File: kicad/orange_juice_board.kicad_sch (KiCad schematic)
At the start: 62 parts, among them J10 PWM_OUT1, J11 CONN_UART, J12 PWM_OUT2, J13 FAN_12/24v, J15 PWM_OUT3, J2 DC_INPUT, J3 CONN_ADXL345, J4 OrangePi Zero GPIO PINs, J5 Conn_MAX31865, J7 OrangePi Zero Function Interf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, J8 FAN_5v, J9 PWR_5v, Q1 AO4407A, Q2 AO3400A, Q3 AO3400A, Q4 AO3400A, U1 MP2315GJ-Z

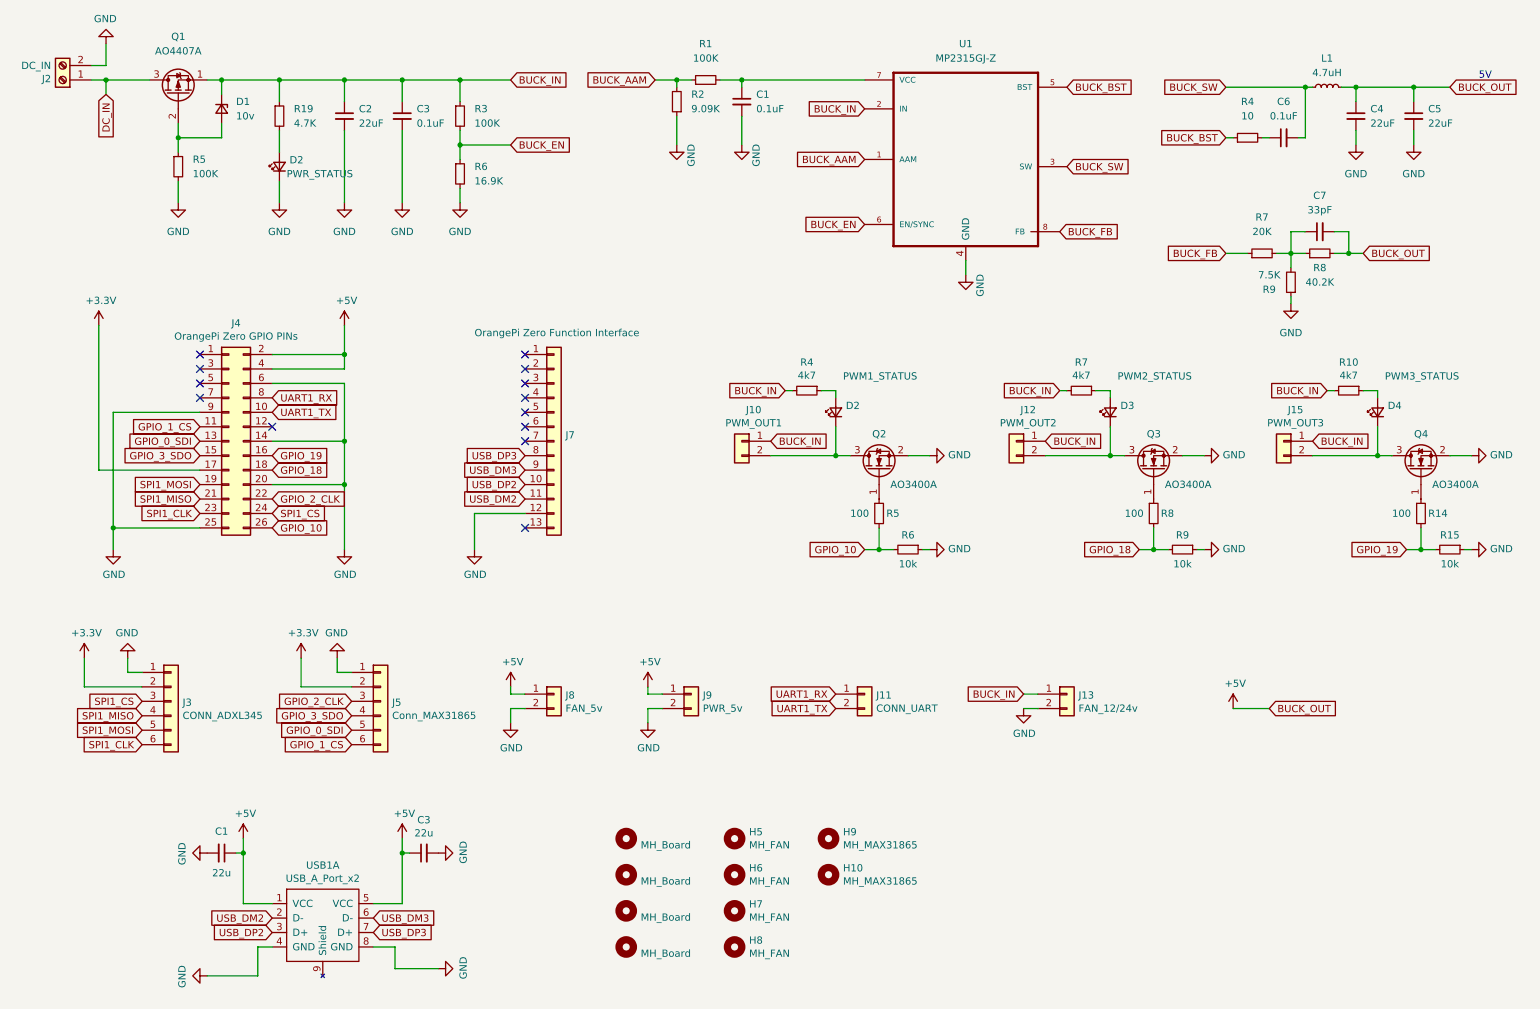
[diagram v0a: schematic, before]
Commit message: update v0.6
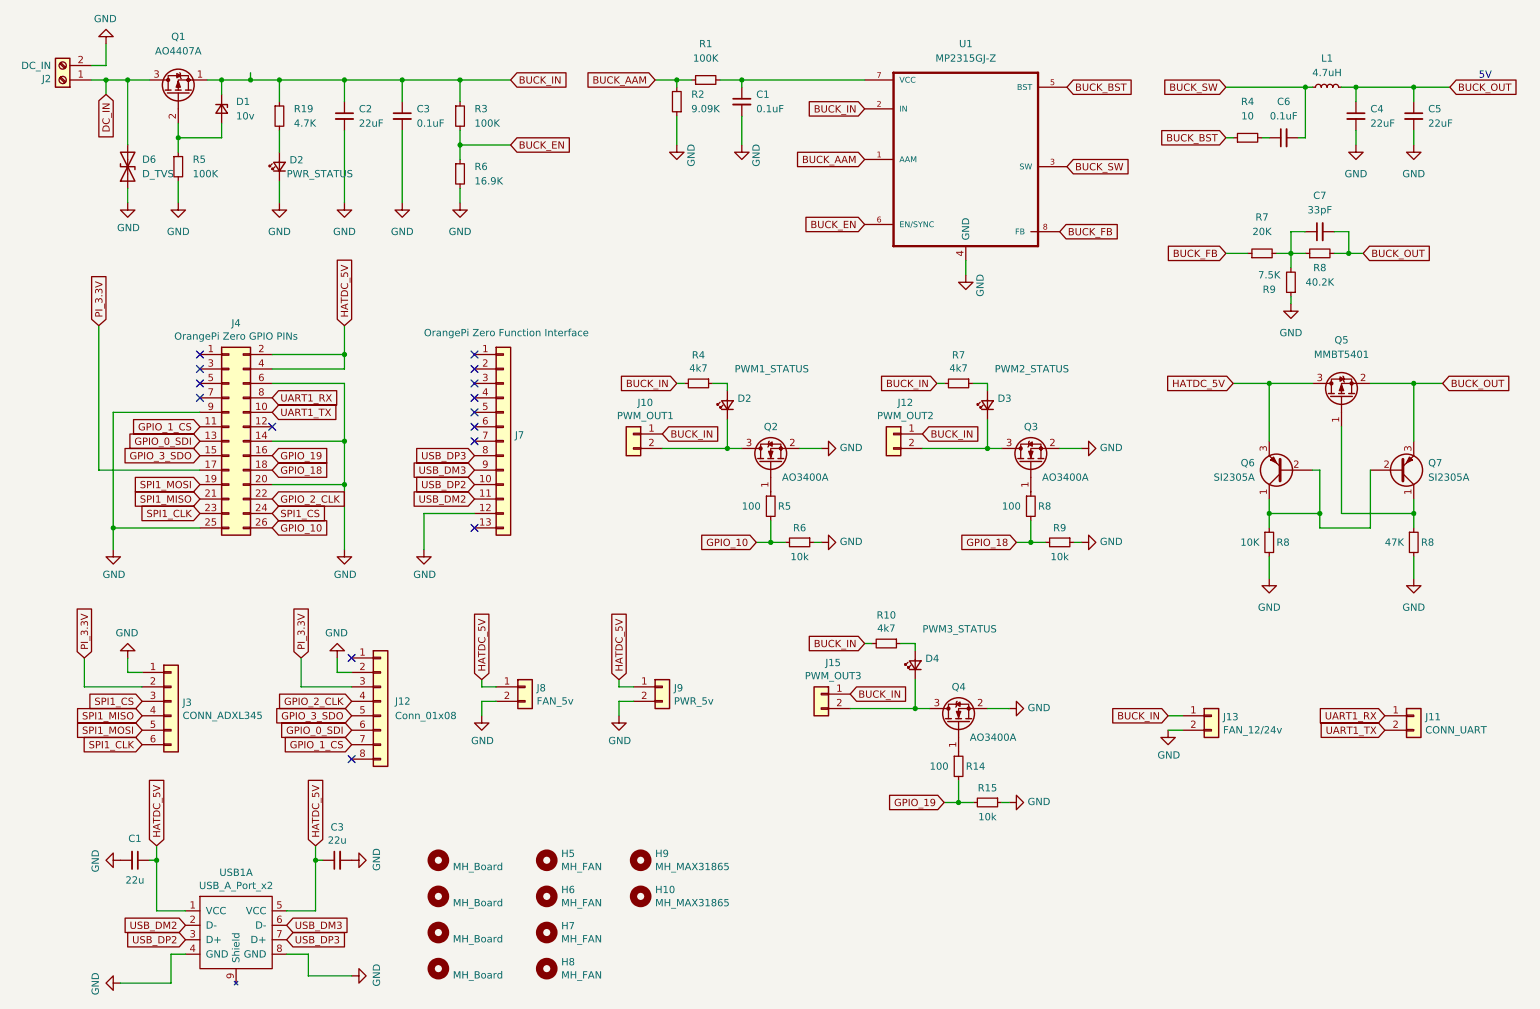
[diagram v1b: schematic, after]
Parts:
- removed J5: Conn_MAX31865, Connector_PinSocket_2.54mm:PinSocket_1x06_P2.54mm_Vertical, symbol orange_juice_board-rescue:Conn_01x06-Connector_Generic-OrangePiZeroExtentionBoa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
- added D6: D_TVS, Diode_SMD:D_SMB, symbol Device:D_TVS
- added J12: Conn_01x08, Connector_PinSocket_2.54mm:PinSocket_1x08_P2.54mm_Vertical, symbol Connector_Generic:Conn_01x08
- added Q5: MMBT5401, Package_TO_SOT_SMD:SOT-23, symbol Device:Q_PMOS_GSD
- added Q6, Q7: SI2305A, Package_TO_SOT_SMD:SOT-23, symbol Device:Q_PNP_CBE
- added R8 (x2): 100, Resistor_SMD:R_0805_2012Metric, symbol orange_juice_board-rescue:R_Small-Device-OrangePiZeroExtentionBoard-rescue-oran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
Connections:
- net DC_IN: now also D6.2 (A2)
- net GND: now also D6.1 (A1), J12.2 (Pin_2), R8.2, R8.2
- net GPIO_0_SDI: now also J12.6 (Pin_6)
- net GPIO_1_CS: now also J12.7 (Pin_7)
- net GPIO_2_CLK: now also J12.4 (Pin_4)
- net GPIO_3_SDO: now also J12.5 (Pin_5)
- net +3V3 renamed PI_3.3V
- net PI_3.3V: now also J12.3 (Pin_3)
- net +5V renamed HATDC_5V
- net HATDC_5V: now also Q5.3 (D), Q6.3 (E); no longer C4.1, C5.1, C7.2, L1.2, R8.2
- new net: Q6.1 (C), Q6.2 (B), Q7.2 (B), R8.1
- new net: Q5.1 (G), Q7.1 (C), R8.1
- new net BUCK_OUT: C4.1, C5.1, C7.2, L1.2, Q5.2 (S), Q7.3 (E), R8.2
- no-connect marks 13 -> 15
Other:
- company: Stone-Jerry -> Stone Lab - Jerry
- title: Orange Pi Zero Adapter -> Orange Juice
- moved on the sheet: C1, C3, D2, D3, D4, H10, H5, H6, H7, H8, H9, J10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
